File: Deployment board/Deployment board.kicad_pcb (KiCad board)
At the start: 4 copper layers, 39 x 62 mm, 32 parts, among them J1 Conn_01x03, J2 Conn_01x03, J3 Conn_01x02, J4 Conn_01x02, J5 Conn_01x02, J6 XT60, J7 Conn_01x02, Q1 IRLR7843, Q2 IRLR7843, Q3 FDD4141, Q4 IRLR7843

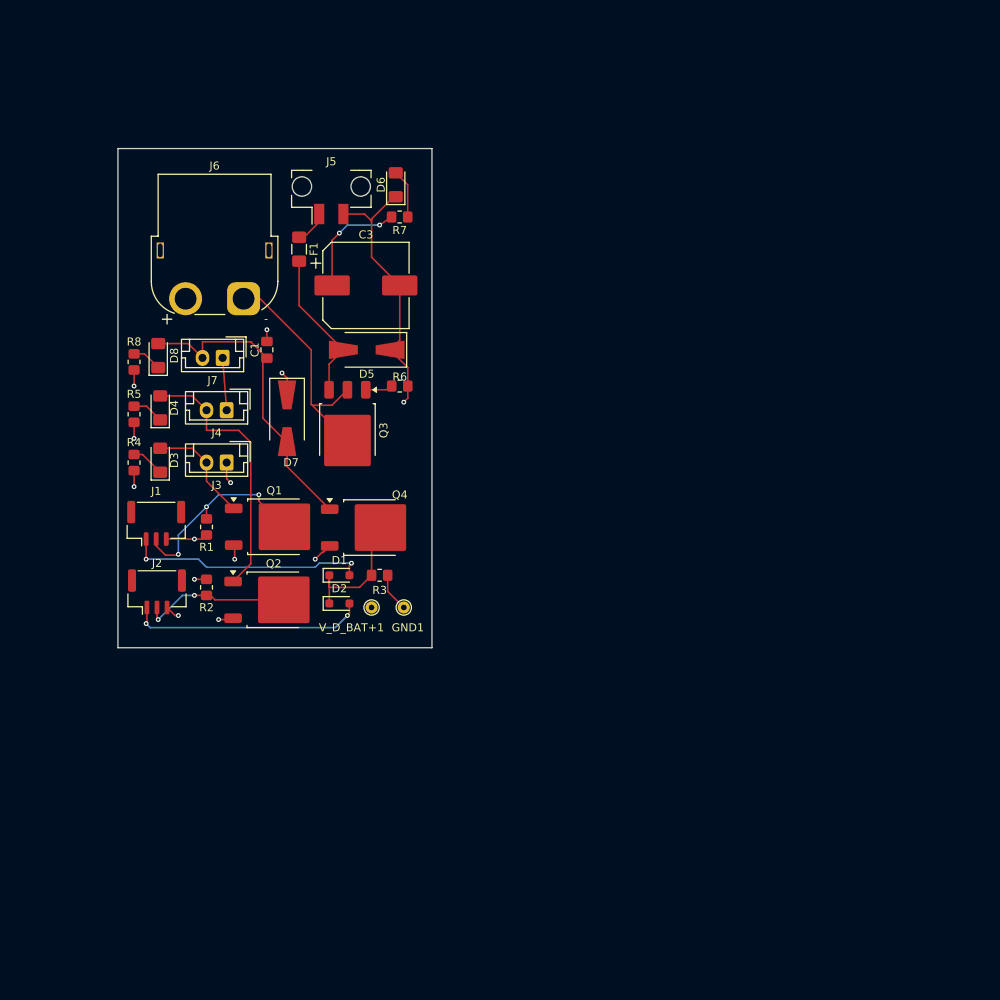
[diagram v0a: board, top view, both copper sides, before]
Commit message: new deployment board
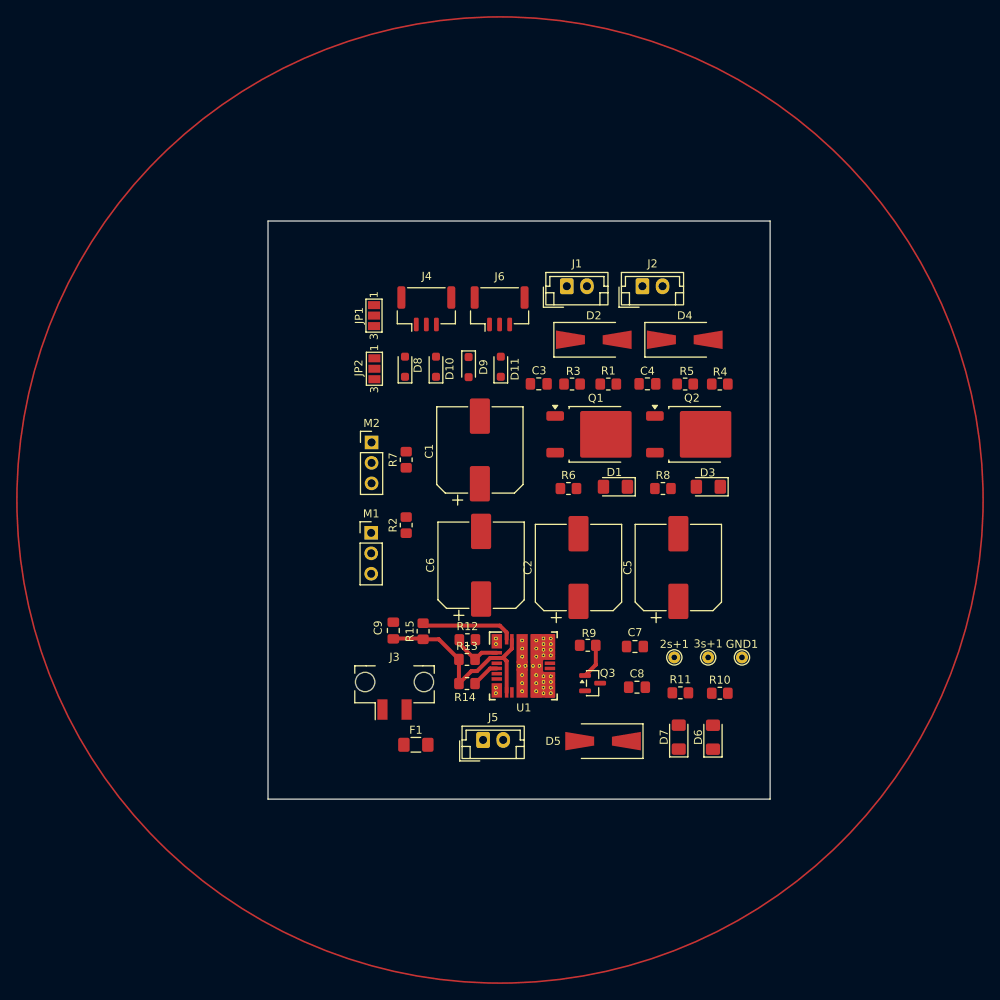
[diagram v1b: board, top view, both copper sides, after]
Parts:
- removed J7: Conn_01x02, Connector_JST:JST_EH_B2B-EH-A_1x02_P2.50mm_Vertical
- removed Q4: IRLR7843, Package_TO_SOT_SMD:TO-252-2
- removed V_D_BAT+1: TestPoint, TestPoint:TestPoint_THTPad_D1.5mm_Drill0.7mm
- added 2s+1: TestPoint, TestPoint:TestPoint_THTPad_D1.5mm_Drill0.7mm, F.Cu at (162.6, 122.2)
- added 3s+1: TestPoint, TestPoint:TestPoint_THTPad_D1.5mm_Drill0.7mm, F.Cu at (166.8, 122.2)
- added C2: 1000u, Capacitor_SMD:CP_Elec_10x14.3, F.Cu at (150.7, 111.0)
- added C4: 100n, Capacitor_SMD:C_0805_2012Metric_Pad1.18x1.45mm_HandSolder, F.Cu at (159.3, 88.2)
- added C5: 1000u, Capacitor_SMD:CP_Elec_10x14.3, F.Cu at (163.1, 111.0)
- added C6: 1000u, Capacitor_SMD:CP_Elec_10x14.3, F.Cu at (138.6, 110.8)
- added C7: 10uF 3.979mOhm, Capacitor_SMD:C_0805_2012Metric_Pad1.18x1.45mm_HandSolder, F.Cu at (157.7, 120.8)
- added C8: 10uF 3.979mOhm, Capacitor_SMD:C_0805_2012Metric_Pad1.18x1.45mm_HandSolder, F.Cu at (158.0, 125.9)
- added C9: 47uF 2.674mOhm Qty=3, Capacitor_SMD:C_0805_2012Metric_Pad1.18x1.45mm_HandSolder, F.Cu at (127.7, 118.9)
- added D10: D_Schottky, Diode_SMD:D_SOD-323_HandSoldering, F.Cu at (133.0, 86.1)
- added D11: D_Schottky, Diode_SMD:D_SOD-323_HandSoldering, F.Cu at (141.1, 86.1)
- added D9: D_Schottky, Diode_SMD:D_SOD-323_HandSoldering, F.Cu at (137.1, 86.1)
- added JP1: Drogue, Jumper:SolderJumper-3_P1.3mm_Open_Pad1.0x1.5mm_NumberLabels, F.Cu at (125.3, 79.8)
- added JP2: Main, Jumper:SolderJumper-3_P1.3mm_Open_Pad1.0x1.5mm_NumberLabels, F.Cu at (125.3, 86.3)
- added M1: Motor_Servo, Connector_PinHeader_2.54mm:PinHeader_1x03_P2.54mm_Vertical, F.Cu at (125.0, 106.7)
- added M2: Motor_Servo, Connector_PinHeader_2.54mm:PinHeader_1x03_P2.54mm_Vertical, F.Cu at (125.0, 95.5)
- added R10: 3.3k, Resistor_SMD:R_0805_2012Metric_Pad1.20x1.40mm_HandSolder, F.Cu at (168.2, 126.7)
- added R11: 3.3k, Resistor_SMD:R_0805_2012Metric_Pad1.20x1.40mm_HandSolder, F.Cu at (163.3, 126.6)
- added R12: 10k, Resistor_SMD:R_0805_2012Metric_Pad1.20x1.40mm_HandSolder, F.Cu at (136.9, 120.0)
- added R13: 866k, Resistor_SMD:R_0805_2012Metric_Pad1.20x1.40mm_HandSolder, F.Cu at (136.8, 122.5)
- added R14: 6.81k, Resistor_SMD:R_0805_2012Metric_Pad1.20x1.40mm_HandSolder, F.Cu at (136.8, 125.5)
- added R15: 34.8k, Resistor_SMD:R_0805_2012Metric_Pad1.20x1.40mm_HandSolder, F.Cu at (131.4, 119.0)
- added R9: 100k, Resistor_SMD:R_0805_2012Metric_Pad1.20x1.40mm_HandSolder, F.Cu at (151.8, 120.7)
- added U1: TPSM84824MOLR, TPSM84824:MOL0024A, F.Cu at (143.8, 123.2)
- C1: value 100n -> 1000u; footprint Capacitor_SMD:C_0805_2012Metric_Pad1.18x1.45mm_HandSolder -> Capacitor_SMD:CP_Elec_10x14.3
- C3: value 1000u -> 100n; footprint Capacitor_SMD:CP_Elec_10x14.3 -> Capacitor_SMD:C_0805_2012Metric_Pad1.18x1.45mm_HandSolder
- D1: value D_Schottky -> Motor; footprint Diode_SMD:D_SOD-323_HandSoldering -> LED_SMD:LED_1206_3216Metric_Pad1.42x1.75mm_HandSolder
- D2: footprint Diode_SMD:D_SOD-323_HandSoldering -> Diode_SMD:D_SMA-SMB_Universal_Handsoldering
- D3: value MFire -> Motor
- D4: value BFire -> D_Schottky; footprint LED_SMD:LED_1206_3216Metric_Pad1.42x1.75mm_HandSolder -> Diode_SMD:D_SMA-SMB_Universal_Handsoldering
- D7: value D_Schottky -> Indicater; footprint Diode_SMD:D_SMA-SMB_Universal_Handsoldering -> LED_SMD:LED_1206_3216Metric_Pad1.42x1.75mm_HandSolder
- D8: value Motor -> D_Schottky; footprint LED_SMD:LED_1206_3216Metric_Pad1.42x1.75mm_HandSolder -> Diode_SMD:D_SOD-323_HandSoldering
- J1, J2: value Conn_01x03 -> Conn_01x02; footprint Connector_JST:JST_GH_BM03B-GHS-TBT_1x03-1MP_P1.25mm_Vertical -> Connector_JST:JST_EH_B2B-EH-A_1x02_P2.50mm_Vertical
- J3: footprint Connector_JST:JST_EH_B2B-EH-A_1x02_P2.50mm_Vertical -> Connector_Molex:Molex_Micro-Fit_3.0_43650-0221_1x02_P3.00mm_Vertical
- J4: value Conn_01x02 -> Conn_01x03; footprint Connector_JST:JST_EH_B2B-EH-A_1x02_P2.50mm_Vertical -> Connector_JST:JST_GH_BM03B-GHS-TBT_1x03-1MP_P1.25mm_Vertical
- J5: footprint Connector_Molex:Molex_Micro-Fit_3.0_43650-0221_1x02_P3.00mm_Vertical -> Connector_JST:JST_EH_B2B-EH-A_1x02_P2.50mm_Vertical
- J6: value XT60 -> Conn_01x03; footprint Connector_AMASS:AMASS_XT60PW-F_1x02_P7.20mm_Horizontal -> Connector_JST:JST_GH_BM03B-GHS-TBT_1x03-1MP_P1.25mm_Vertical
- Q3: footprint Package_TO_SOT_SMD:TO-252-3_TabPin2 -> Package_TO_SOT_SMD:SOT-23
- R1: value 1k -> 100ohm
- R4: value 3.3k -> 100ohm
- R5, R7: value 3.3k -> 1k
- R6: value 100k -> 3.3k
- moved D6 79.1 mm to (167.4, 132.1)
- moved R4 73.4 mm to (168.2, 88.2), turned to 0 degrees
- moved J2 71.2 mm to (158.6, 76.1)
- moved J5 71.0 mm to (138.8, 132.4)
- moved R5 68.6 mm to (163.9, 88.2), turned to 180 degrees
- moved D3 68.2 mm to (166.8, 101.0), turned to 180 degrees
- moved R8 67.5 mm to (161.2, 101.2), turned to 0 degrees
- moved D4 65.7 mm to (163.9, 82.8), turned to 0 degrees
- moved F1 63.2 mm to (130.5, 133.1), turned to 0 degrees
- moved D7 62.7 mm to (163.2, 132.1), turned to 90 degrees
- moved J1 58.9 mm to (149.2, 76.1)
- moved D5 56.8 mm to (153.8, 132.6)
- moved Q2 56.3 mm to (165.2, 94.5)
- moved R1 53.0 mm to (154.4, 88.2), turned to 0 degrees
- moved D2 45.5 mm to (152.6, 82.8)
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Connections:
- C1 pad 1: Net-(D7-A) -> 2s+
- C1 pad 2: V_D_BAT+ -> GND
- C3 pad 1: V_D_BAT+ -> Net-(D2-A)
- C3 pad 2: GND -> 3s+
- D1 pad 1: Net-(D1-K) -> GND
- D1 pad 2: Main_AV_PWM_Servo -> Net-(D1-A)
- D2 pad 1: Net-(D1-K) -> 3s+
- D2 pad 2: Backup_AV_PWM_Servo -> Net-(D2-A)
- D3 pad 1: Net-(D3-K) -> GND
- D4 pad 1: Net-(D4-K) -> 3s+
- D7 pad 1: V_D_BAT+ -> GND
- D8 pad 2: Net-(D7-A) -> Main_AV_PWM_Servo
- F1 pad 1: Net-(J5-Pin_1) -> Net-(J3-Pin_1)
- J1 pad 1: Main_AV_PWM_Servo -> 3s+
- J1 pad 2: Main_AV_FIRE -> Net-(D2-A)
- J2 pad 1: Backup_AV_PWM_Servo -> 3s+
- J2 pad 2: Backup_AV_FIRE -> Net-(D4-A)
- J3 pad 1: V_D_BAT+ -> Net-(J3-Pin_1)
- J3 pad 2: Net-(D3-A) -> GND
- J4 pad 1: V_D_BAT+ -> Main_AV_PWM_Servo
- J4 pad 2: Net-(D4-A) -> Main_AV_FIRE
- J5 pad 1: Net-(J5-Pin_1) -> 3s+
- J5 pad 2: GND -> Net-(D5-A2)
- J6 pad 1: Net-(J6-A) -> Backup_AV_PWM_Servo
- J6 pad 2: V_D_BAT+ -> Backup_AV_FIRE
- Q1 pad 1: Net-(D3-A) -> Net-(D2-A)
- Q1 pad 2: Main_AV_FIRE -> Net-(Q1-G)
- Q2 pad 2: Backup_AV_FIRE -> Net-(Q2-G)
- Q3 pad 2: Net-(J6-A) -> 3s+
- R1 pad 1: Main_AV_FIRE -> Net-(Q1-G)
- R1 pad 2: GND -> 3sMotor2
- R2 pad 1: Backup_AV_FIRE -> 2sServo1
- R3 pad 1: Net-(D1-K) -> Net-(Q1-G)
- R4 pad 1: Net-(D3-K) -> Net-(Q2-G)
- R4 pad 2: GND -> 3sMotor1
- R5 pad 1: Net-(D4-K) -> Net-(Q2-G)
- R6 pad 1: Net-(Q3-G) -> 3s+
- R6 pad 2: GND -> Net-(D1-A)
- R7 pad 1: Net-(D6-A) -> 2sServo2
- R7 pad 2: V_D_BAT+ -> GND
- R8 pad 1: GND -> 3s+
- R8 pad 2: Net-(D8-K) -> Net-(D3-A)
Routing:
- net GND: track 58.9 -> 0.00 mm, vias 10 -> 0
- net Net-(D7-A): track 39.5 -> 0.00 mm
- net Net-(D4-A): track 33.3 -> 0.00 mm
- net Main_AV_PWM_Servo: track 30.2 -> 0.00 mm, vias 2 -> 0
- net Backup_AV_PWM_Servo: track 29.5 -> 0.00 mm, vias 2 -> 0
- net Net-(J6-A): track 29.3 -> 0.00 mm
- net Net-(C9-Pad2): track 0.00 -> 26.7 mm
- net Main_AV_FIRE: track 25.4 -> 0.00 mm, vias 3 -> 0
- net V_D_BAT+: track 19.4 -> 0.00 mm, vias 5 -> 0
- net Net-(D5-A2): track 19.6 -> 0.21 mm
- net Backup_AV_FIRE: track 18.1 -> 0.00 mm, vias 2 -> 0
- net Net-(D1-K): track 15.7 -> 0.00 mm
- net Net-(D3-A): track 13.6 -> 0.00 mm
- net Net-(U1-RT_CLK): track 0.00 -> 11.7 mm
- net Net-(U1-FB): track 0.00 -> 6.30 mm
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- removed copper zone on In2.Cu, net GND
- removed copper zone on In1.Cu, net V_D_BAT+
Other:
- board size 39 x 62 mm -> 62.4 x 71.8 mm

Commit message: jpush
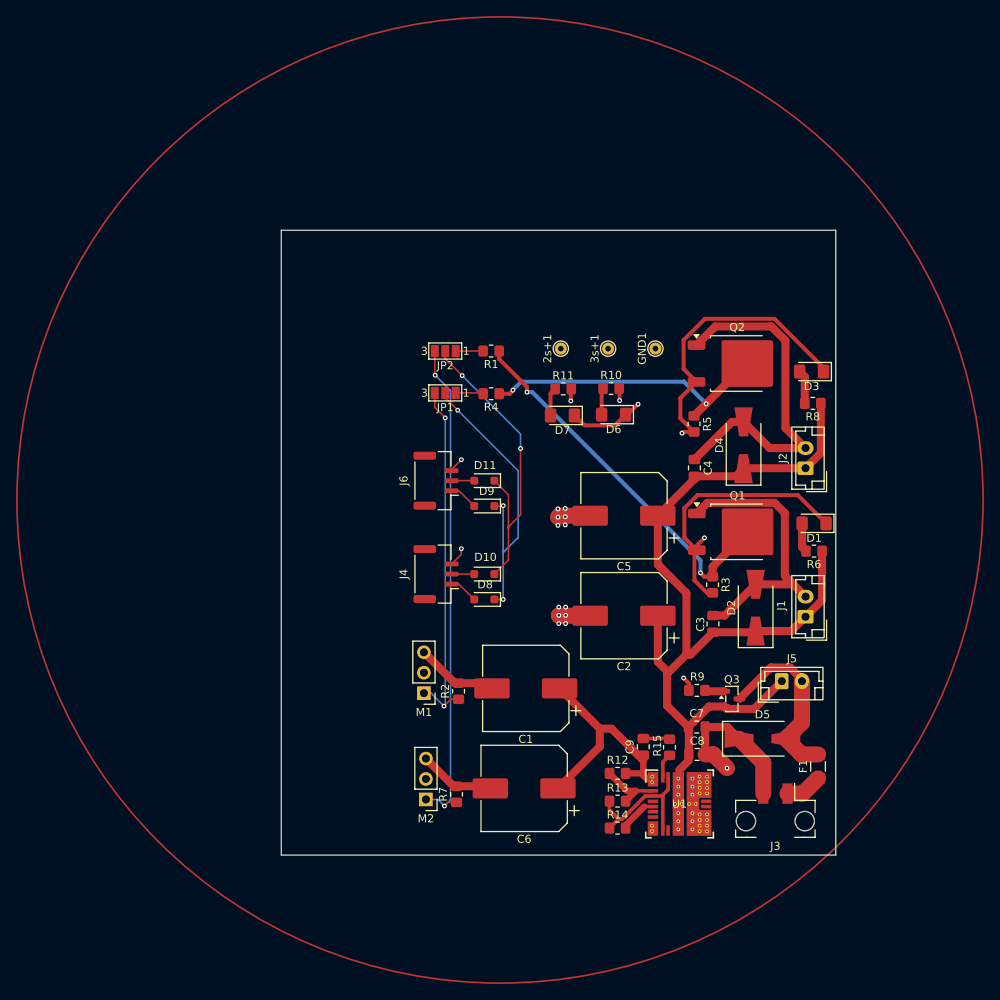
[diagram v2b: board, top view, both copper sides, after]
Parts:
- moved J1 50.6 mm to (178.9, 117.2), turned to 90 degrees
- moved J3 50.2 mm to (175.2, 142.2), turned to 180 degrees
- moved F1 50.0 mm to (180.4, 135.7), turned to 90 degrees
- moved M2 44.9 mm to (131.8, 139.8), turned to 180 degrees
- moved D7 42.5 mm to (148.7, 92.2), turned to 180 degrees
- moved R7 42.0 mm to (135.6, 139.2), turned to 90 degrees
- moved D6 41.9 mm to (155.1, 92.0), turned to 180 degrees
- moved 2s+1 40.9 mm to (148.5, 83.8), turned to 90 degrees
- moved R11 40.5 mm to (148.8, 88.8)
- moved 3s+1 40.3 mm to (154.4, 83.8), turned to 90 degrees
- moved R10 40.2 mm to (154.8, 88.8)
- moved GND1 39.8 mm to (160.2, 83.8), turned to 90 degrees
- moved D2 38.9 mm to (172.7, 116.0), turned to 90 degrees
- moved J5 37.8 mm to (175.9, 125.2)
- moved C3 36.8 mm to (167.4, 118.0), turned to -90 degrees
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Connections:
- C9 pad 2: Net-(C9-Pad2) -> GND
- R13 pad 1: Net-(C9-Pad2) -> GND
- R14 pad 1: Net-(C9-Pad2) -> GND
- R15 pad 1: Net-(C9-Pad2) -> GND
- U1 pad 23: Net-(C9-Pad2) -> GND
- U1 pad 3: Net-(C9-Pad2) -> GND
- U1 pad 9: Net-(C9-Pad2) -> GND
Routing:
- net GND: track 0.00 -> 154.9 mm, vias 0 -> 19
- net 3s+: track 0.00 -> 114.5 mm, vias 0 -> 1
- net 2sServo2: track 0.00 -> 61.9 mm, vias 0 -> 2
- net Net-(Q1-G): track 0.00 -> 47.4 mm, vias 0 -> 2
- net 2sServo1: track 0.00 -> 44.8 mm, vias 0 -> 2
- net Net-(D4-A): track 0.00 -> 44.2 mm
- net Net-(D10-K): track 0.00 -> 39.6 mm, vias 0 -> 2
- net Net-(D8-K): track 0.00 -> 38.3 mm, vias 0 -> 3
- net (no net): track 0.00 -> 37.2 mm
- net Net-(Q2-G): track 0.00 -> 36.7 mm, vias 0 -> 2
- net Net-(D2-A): track 0.00 -> 35.0 mm
- net 2s+: track 0.00 -> 30.7 mm, vias 0 -> 1
- net Net-(C9-Pad2): track 26.7 -> 0.00 mm
- net Net-(D5-A2): track 0.21 -> 22.8 mm
- net Net-(U1-RT_CLK): track 11.7 -> 3.08 mm
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- added copper zone on In1.Cu, net 2s+
- added copper zone on In1.Cu, net 3s+
- added copper zone on In2.Cu, net GND
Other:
- board size 62.4 x 71.8 mm -> 68.9 x 77.6 mm
